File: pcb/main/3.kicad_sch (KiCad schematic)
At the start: 10 parts, among them U5 AP63203WU-7

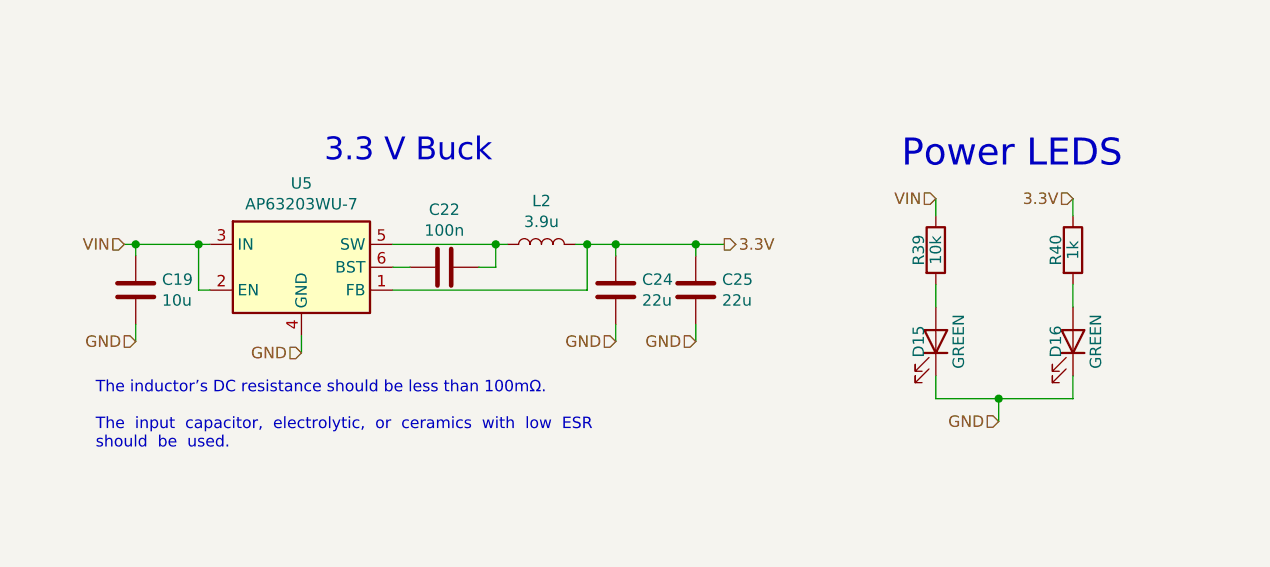
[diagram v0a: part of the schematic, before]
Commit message: feat: updated BOM information
Some components are still without MNF and Seller information
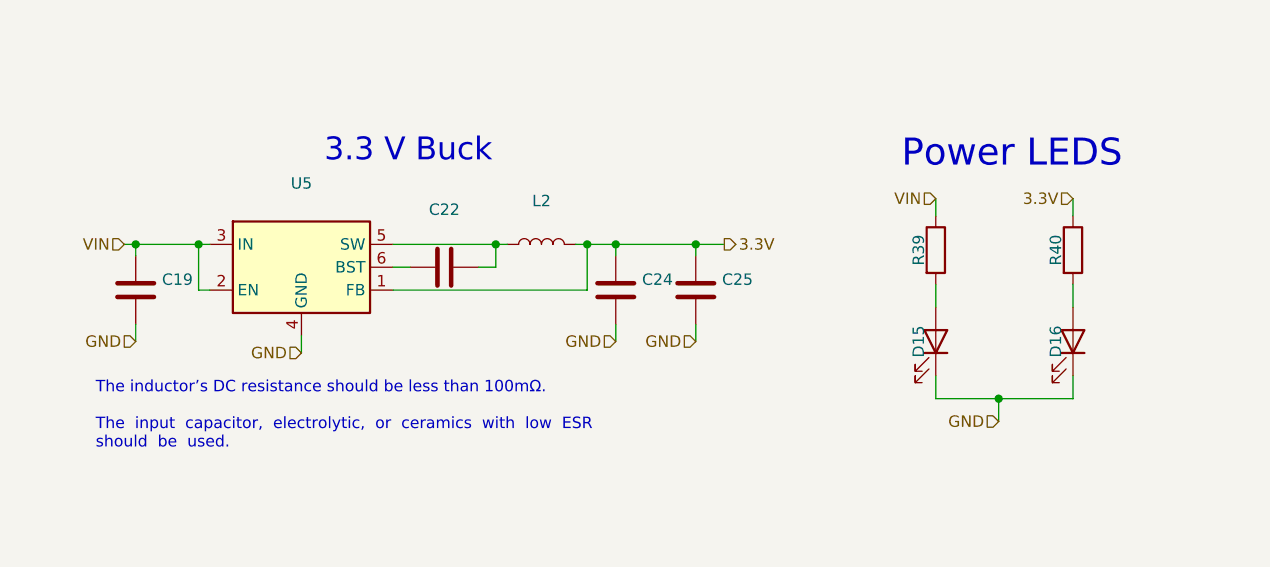
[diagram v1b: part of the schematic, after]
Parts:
- C19: value 10u -> (none); footprint Capacitor_SMD:C_0805_2012Metric_Pad1.18x1.45mm_HandSolder -> (none)
- C22: value 100n -> (none); footprint Capacitor_SMD:C_0805_2012Metric_Pad1.18x1.45mm_HandSolder -> (none)
- C24, C25: value 22u -> (none); footprint Capacitor_SMD:C_0805_2012Metric_Pad1.15x1.40mm_HandSolder -> (none)
- D15, D16: value GREEN -> (none); footprint LED_SMD:LED_0805_2012Metric_Pad1.15x1.40mm_HandSolder -> (none)
- L2: value 3.9u -> (none); footprint Inductor_SMD:L_Taiyo-Yuden_NR-24xx_HandSoldering -> (none); MFN (none) -> Bourns; MFP (none) -> SDR0403-3R9ML; S1PL (none) -> https://www.mouser.com/ProductDetail/652-SDR0403-3R9ML; S1PN (none) -> 652-SDR0403-3R9ML
- R39: value 10k -> (none); footprint Resistor_SMD:R_0805_2012Metric_Pad1.20x1.40mm_HandSolder -> (none)
- R40: value 1k -> (none); footprint Resistor_SMD:R_0805_2012Metric_Pad1.15x1.40mm_HandSolder -> (none); MFN (none) -> KOA Speer; MFP (none) -> RK73H2ATTD1001F; S1PL (none) -> https://www.mouser.com/ProductDetail/KOA-Speer/RK73H2ATTD10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; S1PN (none) -> 660-RK73H2ATTD1001F
- U5: value AP63203WU-7 -> (none); footprint Package_TO_SOT_SMD:TSOT-23-6 -> (none)
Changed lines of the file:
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@@
     (in_bom yes) (on_board yes)
     (property "Reference" "R39" (id 0) (at 172.085 95.885 90))
-    (property "Value" "10k" (id 1) (at 173.99 95.885 90))
-    (property "Footprint" "Resistor_SMD:R_0805_2012Metric_Pad1.20x1.40mm_HandSolder" (id 2) (at 172.212 95.885 90)
+    (property "Value" "" (id 1) (at 173.99 95.885 90))
+    (property "Footprint" "" (id 2) (at 172.212 95.885 90)
       (effects (font (size 1.27 1.27)) hide)
     )
@@
     (in_bom yes) (on_board yes)
     (property "Reference" "R40" (id 0) (at 187.325 95.885 90))
-    (property "Value" "1k" (id 1) (at 189.23 95.885 90))
-    (property "Footprint" "Resistor_SMD:R_0805_2012Metric_Pad1.15x1.40mm_HandSolder" (id 2) (at 187.452 95.885 90)
-      (effects (font (size 1.27 1.27)) hide)
-    )
-    (property "Datasheet" "~" (id 3) (at 189.23 95.885 0)
+    (property "Value" "" (id 1) (at 189.23 95.885 90))
+    (property "Footprint" "" (id 2) (at 187.452 95.885 90)
+      (effects (font (size 1.27 1.27)) hide)
+    )
+    (property "Datasheet" "https://www.mouser.com/datasheet/2/219/RK73H-1825326.pdf" (id 3) (at 189.23 95.885 0)
+      (effects (font (size 1.27 1.27)) hide)
+    )
+    (property "Description" "Thick Film Resistors - SMD 1/4watts 1Kohms 1% " (id 4) (at 189.23 95.885 0)
+      (effects (font (size 1.27 1.27)) hide)
+    )
+    (property "MFN" "KOA Speer " (id 5) (at 189.23 95.885 0)
+      (effects (font (size 1.27 1.27)) hide)
+    )
+    (property "MFP" "RK73H2ATTD1001F " (id 6) (at 189.23 95.885 0)
+      (effects (font (size 1.27 1.27)) hide)
+    )
+    (property "S1PL" "https://www.mouser.com/ProductDetail/KOA-Speer/RK73H2ATTD1001F?qs=sGAEpiMZZMtlubZbdhIBIHMXi0pPDQ96wRIUy6HwZNc%3D" (id 7) (at 189.23 95.885 0)
+      (effects (font (size 1.27 1.27)) hide)
+    )
+    (property "S1PN" "660-RK73H2ATTD1001F " (id 8) (at 189.23 95.885 0)
       (effects (font (size 1.27 1.27)) hide)
     )
@@
     (in_bom yes) (on_board yes)
     (property "Reference" "D15" (id 0) (at 172.085 106.045 0))
-    (property "Value" "GREEN" (id 1) (at 176.53 106.045 0))
-    (property "Footprint" "LED_SMD:LED_0805_2012Metric_Pad1.15x1.40mm_HandSolder" (id 2) (at 173.99 106.045 0)
+    (property "Value" "" (id 1) (at 176.53 106.045 0))
+    (property "Footprint" "" (id 2) (at 173.99 106.045 0)
       (effects (font (size 1.27 1.27)) hide)
     )
@@
     (in_bom yes) (on_board yes)
     (property "Reference" "D16" (id 0) (at 187.325 106.045 0))
-    (property "Value" "GREEN" (id 1) (at 191.77 106.045 0))
-    (property "Footprint" "LED_SMD:LED_0805_2012Metric_Pad1.15x1.40mm_HandSolder" (id 2) (at 189.23 106.045 0)
+    (property "Value" "" (id 1) (at 191.77 106.045 0))
+    (property "Footprint" "" (id 2) (at 189.23 106.045 0)
       (effects (font (size 1.27 1.27)) hide)
     )
@@
     (in_bom yes) (on_board yes)
     (property "Reference" "U5" (id 0) (at 103.505 88.4682 0))
-    (property "Value" "AP63203WU-7" (id 1) (at 103.505 90.7796 0))
-    (property "Footprint" "Package_TO_SOT_SMD:TSOT-23-6" (id 2) (at 103.505 120.65 0)
+    (property "Value" "" (id 1) (at 103.505 90.7796 0))
+    (property "Footprint" "" (id 2) (at 103.505 120.65 0)
       (effects (font (size 1.27 1.27)) hide)
     )
@@
       (effects (font (size 1.27 1.27)) (justify left))
     )
-    (property "Value" "10u" (id 1) (at 88.011 101.473 0)
+    (property "Value" "" (id 1) (at 88.011 101.473 0)
       (effects (font (size 1.27 1.27)) (justify left))
     )
-    (property "Footprint" "Capacitor_SMD:C_0805_2012Metric_Pad1.18x1.45mm_HandSolder" (id 2) (at 86.0552 104.14 0)
+    (property "Footprint" "" (id 2) (at 86.0552 104.14 0)
       (effects (font (size 1.27 1.27)) hide)
     )
@@
     (in_bom yes) (on_board yes)
     (property "Reference" "C22" (id 0) (at 119.38 91.3892 90))
-    (property "Value" "100n" (id 1) (at 119.38 93.7006 90))
-    (property "Footprint" "Capacitor_SMD:C_0805_2012Metric_Pad1.18x1.45mm_HandSolder" (id 2) (at 115.57 98.7552 0)
+    (property "Value" "" (id 1) (at 119.38 93.7006 90))
+    (property "Footprint" "" (id 2) (at 115.57 98.7552 0)
       (effects (font (size 1.27 1.27)) hide)
     )
@@
     (in_bom yes) (on_board yes)
     (property "Reference" "L2" (id 0) (at 130.175 90.424 90))
-    (property "Value" "3.9u" (id 1) (at 130.175 92.7354 90))
-    (property "Footprint" "Inductor_SMD:L_Taiyo-Yuden_NR-24xx_HandSoldering" (id 2) (at 130.175 95.25 0)
-      (effects (font (size 1.27 1.27)) hide)
-    )
-    (property "Datasheet" "~" (id 3) (at 130.175 95.25 0)
+    (property "Value" "" (id 1) (at 130.175 92.7354 90))
+    (property "Footprint" "" (id 2) (at 130.175 95.25 0)
+      (effects (font (size 1.27 1.27)) hide)
+    )
+    (property "Datasheet" "https://www.mouser.com/datasheet/2/54/sdr0403-1391311.pdf" (id 3) (at 130.175 95.25 0)
+      (effects (font (size 1.27 1.27)) hide)
+    )
+    (property "Description" "Fixed Inductors 3.9uH 20% SMD 0403 " (id 4) (at 130.175 95.25 0)
+      (effects (font (size 1.27 1.27)) hide)
+    )
+    (property "MFN" "Bourns " (id 5) (at 130.175 95.25 0)
+      (effects (font (size 1.27 1.27)) hide)
+    )
+    (property "MFP" "SDR0403-3R9ML " (id 6) (at 130.175 95.25 0)
+      (effects (font (size 1.27 1.27)) hide)
+    )
+    (property "S1PL" "https://www.mouser.com/ProductDetail/652-SDR0403-3R9ML" (id 7) (at 130.175 95.25 0)
+      (effects (font (size 1.27 1.27)) hide)
+    )
+    (property "S1PN" "652-SDR0403-3R9ML " (id 8) (at 130.175 95.25 0)
       (effects (font (size 1.27 1.27)) hide)
     )
@@
       (effects (font (size 1.27 1.27)) (justify right))
     )
-    (property "Value" "22u" (id 1) (at 141.351 101.473 0)
-      (effects (font (size 1.27 1.27)) (justify right))
-    )
-    (property "Footprint" "Capacitor_SMD:C_0805_2012Metric_Pad1.15x1.40mm_HandSolder" (id 2) (at 137.4648 96.52 0)
+    (property "Value" "" (id 1) (at 141.351 101.473 0)
+      (effects (font (size 1.27 1.27)) (justify right))
+    )
+    (property "Footprint" "" (id 2) (at 137.4648 96.52 0)
       (effects (font (size 1.27 1.27)) hide)
     )
@@
       (effects (font (size 1.27 1.27)) (justify right))
     )
-    (property "Value" "22u" (id 1) (at 150.241 101.473 0)
-      (effects (font (size 1.27 1.27)) (justify right))
-    )
-    (property "Footprint" "Capacitor_SMD:C_0805_2012Metric_Pad1.15x1.40mm_HandSolder" (id 2) (at 146.3548 96.52 0)
-      (effects (font (size 1.27 1.27)) hide)
-    )
+    (property "Value" "" (id 1) (at 150.241 101.473 0)
+      (effects (font (size 1.27 1.27)) (justify right))
+    )
+    (property "Footprint" "" (id 2) (at 146.3548 96.52 0)
+      (effects (font (size 1.27 1.27)) hide)
+    )

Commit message: feat: updated BOM
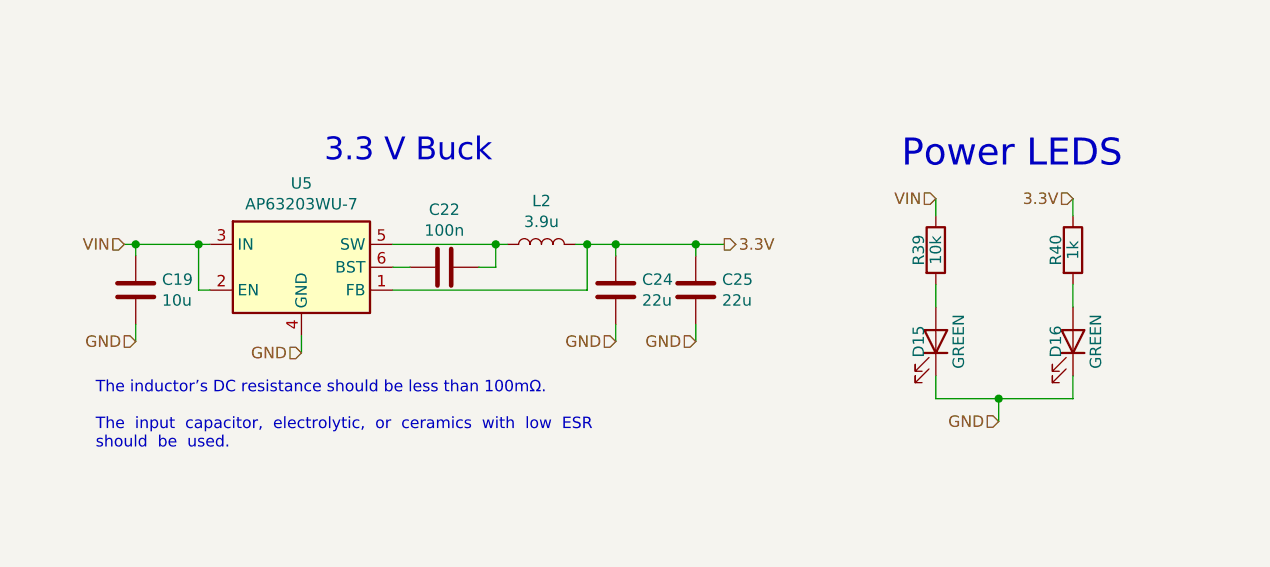
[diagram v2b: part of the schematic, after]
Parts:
- C19: value (none) -> 10u; footprint (none) -> Capacitor_SMD:C_0805_2012Metric_Pad1.18x1.45mm_HandSolder
- C22: value (none) -> 100n; footprint (none) -> Capacitor_SMD:C_0805_2012Metric_Pad1.18x1.45mm_HandSolder
- C24, C25: value (none) -> 22u; footprint (none) -> Capacitor_SMD:C_0805_2012Metric_Pad1.18x1.45mm_HandSolder
- D15, D16: value (none) -> GREEN; footprint (none) -> LED_SMD:LED_0805_2012Metric_Pad1.15x1.40mm_HandSolder
- L2: value (none) -> 3.9u
- R39: value (none) -> 10k
- R40: value (none) -> 1k
- U5: value (none) -> AP63203WU-7
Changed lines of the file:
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@@
     (in_bom yes) (on_board yes)
     (property "Reference" "R39" (id 0) (at 172.085 95.885 90))
-    (property "Value" "" (id 1) (at 173.99 95.885 90))
+    (property "Value" "10k" (id 1) (at 173.99 95.885 90))
     (property "Footprint" "" (id 2) (at 172.212 95.885 90)
       (effects (font (size 1.27 1.27)) hide)
@@
     (in_bom yes) (on_board yes)
     (property "Reference" "R40" (id 0) (at 187.325 95.885 90))
-    (property "Value" "" (id 1) (at 189.23 95.885 90))
+    (property "Value" "1k" (id 1) (at 189.23 95.885 90))
     (property "Footprint" "" (id 2) (at 187.452 95.885 90)
       (effects (font (size 1.27 1.27)) hide)
@@
     (in_bom yes) (on_board yes)
     (property "Reference" "D15" (id 0) (at 172.085 106.045 0))
-    (property "Value" "" (id 1) (at 176.53 106.045 0))
-    (property "Footprint" "" (id 2) (at 173.99 106.045 0)
+    (property "Value" "GREEN" (id 1) (at 176.53 106.045 0))
+    (property "Footprint" "LED_SMD:LED_0805_2012Metric_Pad1.15x1.40mm_HandSolder" (id 2) (at 173.99 106.045 0)
       (effects (font (size 1.27 1.27)) hide)
     )
@@
     (in_bom yes) (on_board yes)
     (property "Reference" "D16" (id 0) (at 187.325 106.045 0))
-    (property "Value" "" (id 1) (at 191.77 106.045 0))
-    (property "Footprint" "" (id 2) (at 189.23 106.045 0)
+    (property "Value" "GREEN" (id 1) (at 191.77 106.045 0))
+    (property "Footprint" "LED_SMD:LED_0805_2012Metric_Pad1.15x1.40mm_HandSolder" (id 2) (at 189.23 106.045 0)
       (effects (font (size 1.27 1.27)) hide)
     )
@@
     (in_bom yes) (on_board yes)
     (property "Reference" "U5" (id 0) (at 103.505 88.4682 0))
-    (property "Value" "" (id 1) (at 103.505 90.7796 0))
+    (property "Value" "AP63203WU-7" (id 1) (at 103.505 90.7796 0))
     (property "Footprint" "" (id 2) (at 103.505 120.65 0)
       (effects (font (size 1.27 1.27)) hide)
@@
       (effects (font (size 1.27 1.27)) (justify left))
     )
-    (property "Value" "" (id 1) (at 88.011 101.473 0)
+    (property "Value" "10u" (id 1) (at 88.011 101.473 0)
       (effects (font (size 1.27 1.27)) (justify left))
     )
-    (property "Footprint" "" (id 2) (at 86.0552 104.14 0)
+    (property "Footprint" "Capacitor_SMD:C_0805_2012Metric_Pad1.18x1.45mm_HandSolder" (id 2) (at 86.0552 104.14 0)
       (effects (font (size 1.27 1.27)) hide)
     )
@@
     (in_bom yes) (on_board yes)
     (property "Reference" "C22" (id 0) (at 119.38 91.3892 90))
-    (property "Value" "" (id 1) (at 119.38 93.7006 90))
-    (property "Footprint" "" (id 2) (at 115.57 98.7552 0)
+    (property "Value" "100n" (id 1) (at 119.38 93.7006 90))
+    (property "Footprint" "Capacitor_SMD:C_0805_2012Metric_Pad1.18x1.45mm_HandSolder" (id 2) (at 115.57 98.7552 0)
       (effects (font (size 1.27 1.27)) hide)
     )
@@
     (in_bom yes) (on_board yes)
     (property "Reference" "L2" (id 0) (at 130.175 90.424 90))
-    (property "Value" "" (id 1) (at 130.175 92.7354 90))
+    (property "Value" "3.9u" (id 1) (at 130.175 92.7354 90))
     (property "Footprint" "" (id 2) (at 130.175 95.25 0)
       (effects (font (size 1.27 1.27)) hide)
@@
       (effects (font (size 1.27 1.27)) (justify right))
     )
-    (property "Value" "" (id 1) (at 141.351 101.473 0)
-      (effects (font (size 1.27 1.27)) (justify right))
-    )
-    (property "Footprint" "" (id 2) (at 137.4648 96.52 0)
+    (property "Value" "22u" (id 1) (at 141.351 101.473 0)
+      (effects (font (size 1.27 1.27)) (justify right))
+    )
+    (property "Footprint" "Capacitor_SMD:C_0805_2012Metric_Pad1.18x1.45mm_HandSolder" (id 2) (at 137.4648 96.52 0)
       (effects (font (size 1.27 1.27)) hide)
     )
@@
       (effects (font (size 1.27 1.27)) (justify right))
     )
-    (property "Value" "" (id 1) (at 150.241 101.473 0)
-      (effects (font (size 1.27 1.27)) (justify right))
-    )
-    (property "Footprint" "" (id 2) (at 146.3548 96.52 0)
-      (effects (font (size 1.27 1.27)) hide)
-    )
+    (property "Value" "22u" (id 1) (at 150.241 101.473 0)
+      (effects (font (size 1.27 1.27)) (justify right))
+    )
+    (property "Footprint" "Capacitor_SMD:C_0805_2012Metric_Pad1.18x1.45mm_HandSolder" (id 2) (at 146.3548 96.52 0)
+      (effects (font (size 1.27 1.27)) hide)
+    )
